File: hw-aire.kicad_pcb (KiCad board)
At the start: 2 copper layers, 78 x 60 mm, 61 parts, among them J1 Conn_01x02_Pin, J3 Screw_Terminal_01x12, J4 Conn_01x05_Pin, J5 Conn_01x02_Pin, K1 JRC-21F(4100), K2 JRC-21F(4100), K3 JRC-21F(4100), Q1 PMBT3904235, Q2 PMBT3904235, Q3 PMBT3904235, Q4 PMBT3904235, SW1 SW_Push, U1 SHT4x, U2 NCP1117-3.3_SOT223, U3 HLK-2M05, U4 BMP581, U5 ESP-12E, U6 PCA9536D

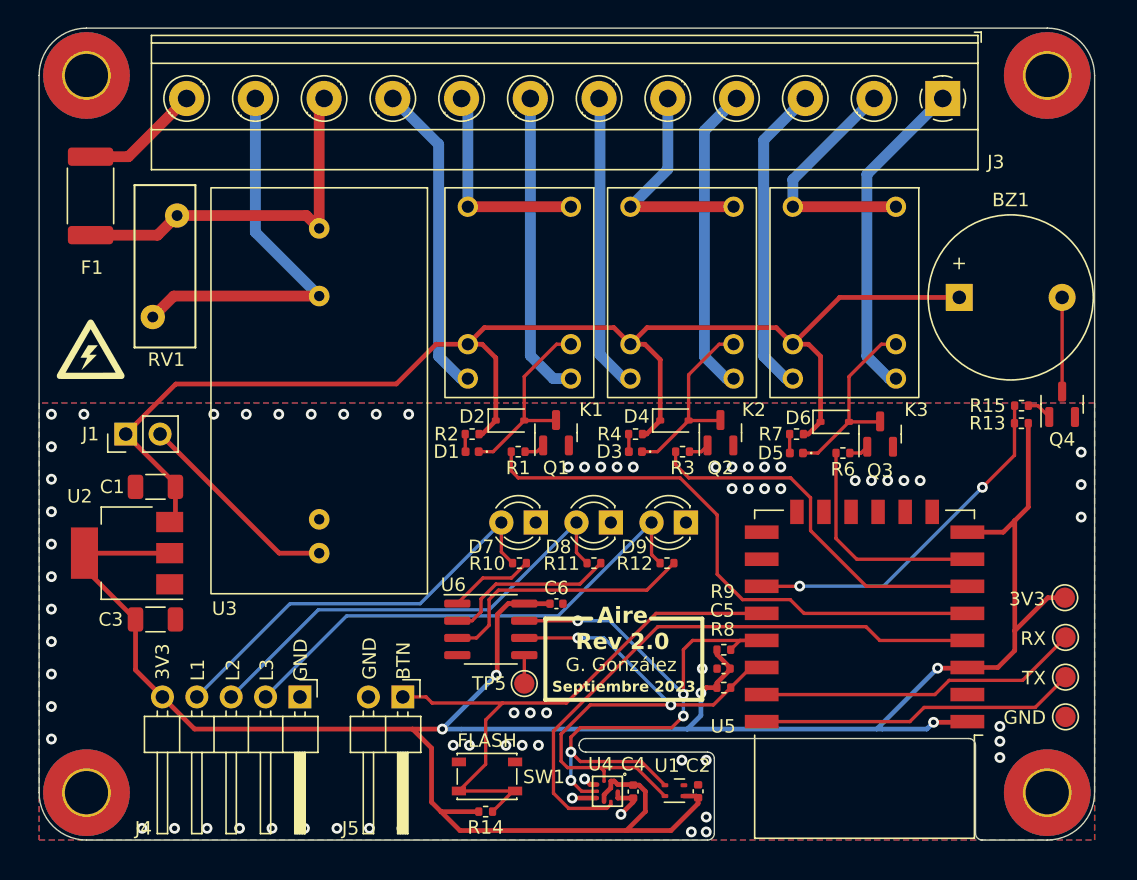
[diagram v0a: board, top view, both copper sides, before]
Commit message: Finish PCB rev 3.0
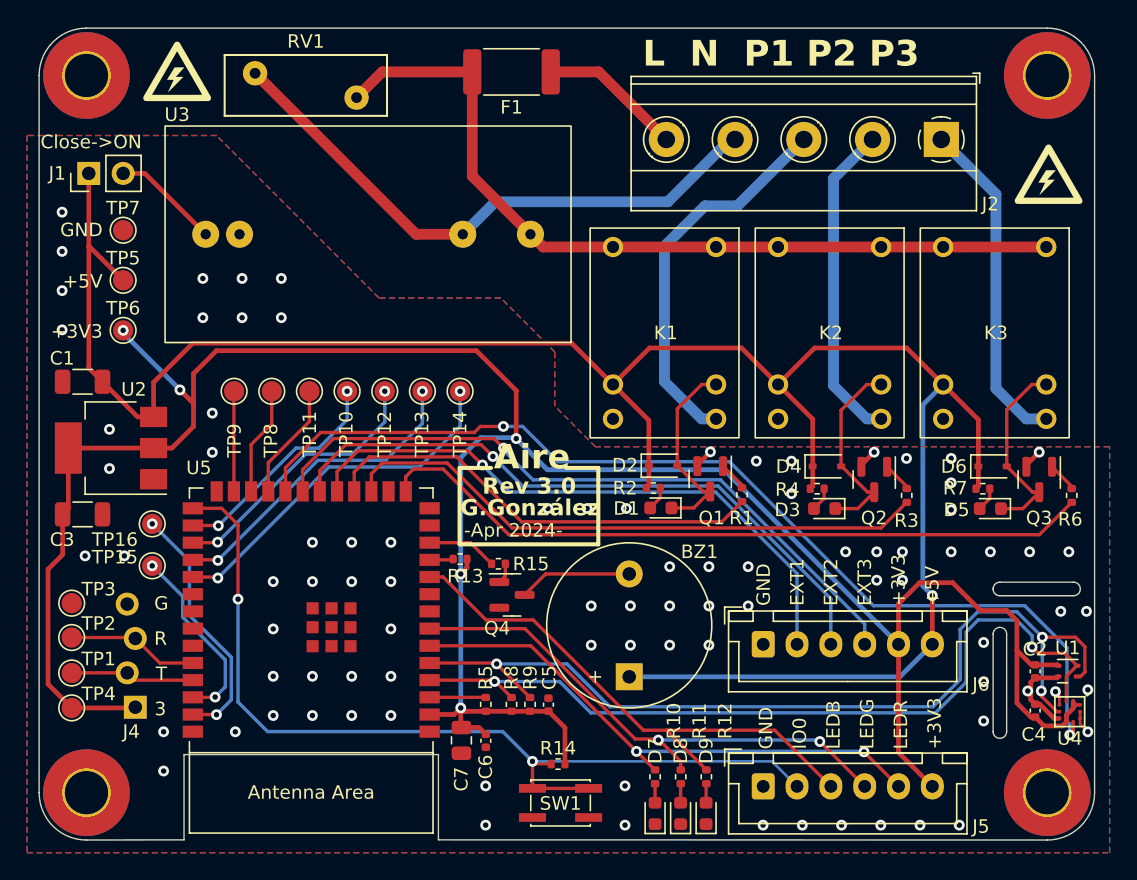
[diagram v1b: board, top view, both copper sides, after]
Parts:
- removed the G*** at (110.6, 90.6)
- removed the G*** at (121.6, 88.2)
- removed J3: Screw_Terminal_01x12, TerminalBlock_Phoenix:TerminalBlock_Phoenix_MKDS-1,5-12-5.08_1x12_P5.08mm_Horizontal
- removed U6: PCA9536D, Package_SO:SOIC-8_3.9x4.9mm_P1.27mm
- added C7: 22u, Capacitor_SMD:C_0805_2012Metric, F.Cu at (138.0, 119.5)
- added G***: LOGO, guille-lib:high_voltage_5mm, F.Cu at (181.4, 77.7)
- added G***: LOGO, guille-lib:high_voltage_5mm, F.Cu at (117.0, 70.1)
- added G***: LOGO, guille-lib:high_voltage, B.Cu at (165.2, 86.9)
- added G***: LOGO, guille-lib:high_voltage, B.Cu at (141.4, 73.1)
- added J2: Screw_Terminal_01x05, TerminalBlock_Phoenix:TerminalBlock_Phoenix_MKDS-1,5-5-5.08_1x05_P5.08mm_Horizontal, F.Cu at (173.5, 75.1)
- added J6: Conn_01x06_Socket, Connector_JST:JST_XH_B6B-XH-A_1x06_P2.50mm_Vertical, F.Cu at (160.3, 112.4)
- added R5: 10k, Resistor_SMD:R_0402_1005Metric, F.Cu at (139.8, 116.8)
- added TP10: TestPoint, TestPoint:TestPoint_Pad_D1.5mm, F.Cu at (129.5, 93.7)
- added TP11: TestPoint, TestPoint:TestPoint_Pad_D1.5mm, F.Cu at (126.8, 93.7)
- added TP12: TestPoint, TestPoint:TestPoint_Pad_D1.5mm, F.Cu at (132.3, 93.7)
- added TP13: TestPoint, TestPoint:TestPoint_Pad_D1.5mm, F.Cu at (135.1, 93.7)
- added TP14: TestPoint, TestPoint:TestPoint_Pad_D1.5mm, F.Cu at (137.9, 93.7)
- added TP15: TestPoint, TestPoint:TestPoint_Pad_D1.5mm, F.Cu at (115.2, 106.6)
- added TP16: TestPoint, TestPoint:TestPoint_Pad_D1.5mm, F.Cu at (115.2, 103.5)
- added TP6: TestPoint, TestPoint:TestPoint_Pad_D1.5mm, F.Cu at (113.0, 89.2)
- added TP7: TestPoint, TestPoint:TestPoint_Pad_D1.5mm, F.Cu at (113.0, 81.8)
- added TP8: TestPoint, TestPoint:TestPoint_Pad_D1.5mm, F.Cu at (124.0, 93.7)
- added TP9: TestPoint, TestPoint:TestPoint_Pad_D1.5mm, F.Cu at (121.2, 93.7)
- D1, D3, D5: footprint LED_SMD:LED_0402_1005Metric -> LED_SMD:LED_0603_1608Metric
- D2, D4, D6: value D -> 1N4448W
- D7, D8, D9: footprint LED_THT:LED_D3.0mm -> LED_SMD:LED_0603_1608Metric
- J4: value Conn_01x05_Pin -> Conn_01x04_Pin; footprint Connector_PinHeader_2.54mm:PinHeader_1x05_P2.54mm_Horizontal -> guille-lib:PinHeaderOffset_1x04_P2.54mm_Vertical
- J5: value Conn_01x02_Pin -> Conn_01x06_Socket; footprint Connector_PinHeader_2.54mm:PinHeader_1x02_P2.54mm_Horizontal -> Connector_JST:JST_XH_B6B-XH-A_1x06_P2.50mm_Vertical
- U5: value ESP-12E -> ESP32-S2-SOLO; footprint RF_Module:ESP-12E -> PCM_Espressif:ESP32-S2-SOLO
- moved TP3 73.9 mm to (109.2, 109.4), turned to 180 degrees
- moved TP4 73.8 mm to (109.2, 117.1), turned to 180 degrees
- moved TP1 73.4 mm to (109.2, 114.5), turned to 180 degrees
- moved TP2 73.4 mm to (109.2, 111.9), turned to 180 degrees
- moved Q4 43.0 mm to (141.7, 108.8), turned to 0 degrees
- moved R13 42.7 mm to (137.9, 106.1)
- moved TP5 42.0 mm to (113.0, 85.5), turned to 180 degrees
- moved U5 41.1 mm to (126.9, 110.6)
- moved R15 40.4 mm to (140.7, 106.5)
- moved BZ1 37.2 mm to (150.4, 114.8), turned to 90 degrees
- moved U4 34.7 mm to (183.0, 117.4)
- moved F1 32.4 mm to (141.7, 70.1), turned to 180 degrees
- moved U1 30.4 mm to (182.8, 114.4), turned to 180 degrees
- moved C4 30.3 mm to (180.4, 117.3), turned to 90 degrees
- moved J5 27.4 mm to (160.3, 122.9), turned to 0 degrees
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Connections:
- D7 pad 2: /LED1R -> Net-(D7-A)
- D8 pad 2: /LED2R -> Net-(D8-A)
- D9 pad 2: /LED3R -> Net-(D9-A)
- J4 pad 1: GND -> +3V3
- J4 pad 2: /LED3R -> /ESP_TX
- J4 pad 3: /LED2R -> /ESP_RX
- J4 pad 4: /LED1R -> GND
- J5 pad 1: /GPIO0 -> GND
- J5 pad 2: GND -> /ESP_IO0
- K1 pad 1: /COM1 -> /LF
- K1 pad 3: /NC1 -> unconnected-(K1-NC-Pad3)
- K1 pad 4: /NO1 -> /P1
- K1 pad 6: /COM1 -> /LF
- K2 pad 1: /COM2 -> /LF
- K2 pad 3: /NC2 -> unconnected-(K2-NC-Pad3)
- K2 pad 4: /NO2 -> /P2
- K2 pad 6: /COM2 -> /LF
- K3 pad 1: /COM3 -> /LF
- K3 pad 3: /NC3 -> unconnected-(K3-NC-Pad3)
- K3 pad 4: /NO3 -> /P3
- K3 pad 6: /COM3 -> /LF
- R10 pad 1: /LED1 -> /LEDR
- R10 pad 2: /LED1R -> Net-(D7-A)
- R11 pad 1: /LED2 -> /LEDG
- R11 pad 2: /LED2R -> Net-(D8-A)
- R12 pad 1: /LED3 -> /LEDB
- R12 pad 2: /LED3R -> Net-(D9-A)
- R13 pad 1: /BUZZ -> Net-(U5-GPIO18/U1RXD/ADC2_CH7/DAC_2/CLK_OUT3)
- R14 pad 1: /GPIO0 -> /ESP_IO0
- SW1 pad 2: /GPIO0 -> /ESP_IO0
- TP1 pad 1: /TX -> /ESP_TX
- TP2 pad 1: /RX -> /ESP_RX
- TP5 pad 1: Net-(U6-IO3) -> +5V
- U5 pad 1: +3V3 -> GND
- U5 pad 10: unconnected-(U5-MISO-Pad10) -> /LEDB
- U5 pad 11: unconnected-(U5-GPIO9-Pad11) -> Net-(U5-GPIO18/U1RXD/ADC2_CH7/DAC_2/CLK_OUT3)
- U5 pad 12: unconnected-(U5-GPIO10-Pad12) -> /BUZZ
- U5 pad 15: GND -> /FAN3
- U5 pad 16: GND -> unconnected-(U5-GPIO46-Pad16)
- U5 pad 17: /BUZZ -> /FAN2
- U5 pad 18: /GPIO0 -> /FAN1
- U5 pad 19: /I2C_SDA -> /EXT1
- U5 pad 2: unconnected-(U5-ADC-Pad2) -> +3V3
- U5 pad 20: /I2C_SCL -> /EXT2
- U5 pad 21: /RX -> /EXT3
- U5 pad 22: /TX -> /BMP_INT
- U5 pad 3: +3V3 -> Net-(U5-EN)
- U5 pad 4: /BMP_INT -> /I2C_SCL
- U5 pad 5: /FAN1 -> /I2C_SDA
- U5 pad 6: /FAN2 -> /LEDR
- U5 pad 7: /FAN3 -> /LEDG
- U5 pad 8: +3V3 -> unconnected-(U5-GPIO15/U0RTS/ADC2_CH4/XTAL_32K_P-Pad8)
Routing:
- net /ESP_IO0: track 0.00 -> 68.9 mm, vias 0 -> 2
- net +5V: track 102.6 -> 162.1 mm, vias 0 -> 1
- net /EXT3: track 0.00 -> 51.4 mm, vias 0 -> 1
- net /EXT2: track 0.00 -> 48.2 mm, vias 0 -> 1
- net /EXT1: track 0.00 -> 45.1 mm, vias 0 -> 1
- net /GPIO0: track 44.0 -> 0.00 mm
- net /LEDR: track 0.00 -> 40.9 mm, vias 0 -> 2
- net /LEDB: track 0.00 -> 40.2 mm
- net /LEDG: track 0.00 -> 39.9 mm, vias 0 -> 2
- net /LED3R: track 37.1 -> 0.00 mm
- net /FAN3: track 16.7 -> 53.5 mm
- net /LED2R: track 34.2 -> 0.00 mm
- net /LF: track 27.6 -> 61.6 mm
- net /BMP_INT: track 43.9 -> 75.1 mm, vias 0 -> 2
- net /LED1R: track 31.2 -> 0.00 mm
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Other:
- outline, holes or cut-outs redrawn
- board text added: "+3V3"
- board text added: "+5V"
- board text added: "-Apr 2024-"
- board text added: "3"
- board text added: "Aire"
- board text added: "Close->ON"
- board text added: "EXT1"
- board text added: "EXT2"
- board text added: "EXT3"
- board text added: "G"
- board text added: "G.González"
- board text added: "IO0"
- board text added: "L N P1 P2 P3"
- board text added: "LEDB"
- board text added: "LEDG"
- board text added: "LEDR"
- board text added: "P3 P2 P1 N L"
- board text added: "R"
- board text added: "Rev 3.0"
- board text added: "T"
- board text removed: "3V3"
- board text removed: "Aire Rev 2.0"
- board text removed: "BTN"
- board text removed: "FLASH"
- board text removed: "G. González"
- board text removed: "Guillermo González"
- board text removed: "L1"
- board text removed: "L2"
- board text removed: "L3"
- board text removed: "RX"
- board text removed: "Septiembre 2023"
- board text removed: "TX"
